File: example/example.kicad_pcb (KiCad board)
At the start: 4 copper layers, 80 x 49 mm, 124 parts, among them J1 USB_B_Micro, J2 Conn_02x10_Odd_Even, J3 Conn_02x10_Odd_Even, J4 Conn_01x02, U1 CY7C68013A-56LTX, U10 DAC081C081CIMK, U11 TPS73101DBV, U12 ADC081C021CIMM, U13 DAC081C081CIMK, U14 TPS73101DBV, U15 TPD3S014, U2 CAT24M01W, U3 CAT24C256W, U4 ICE40UP5K-SG48ITR, U5 FXMA108BQX, U6 FXMA108BQX, U7 LM3880MF-1AF, U8 MIC5355-S4YMME, U9 ADC081C021CIMM, Y1 24M

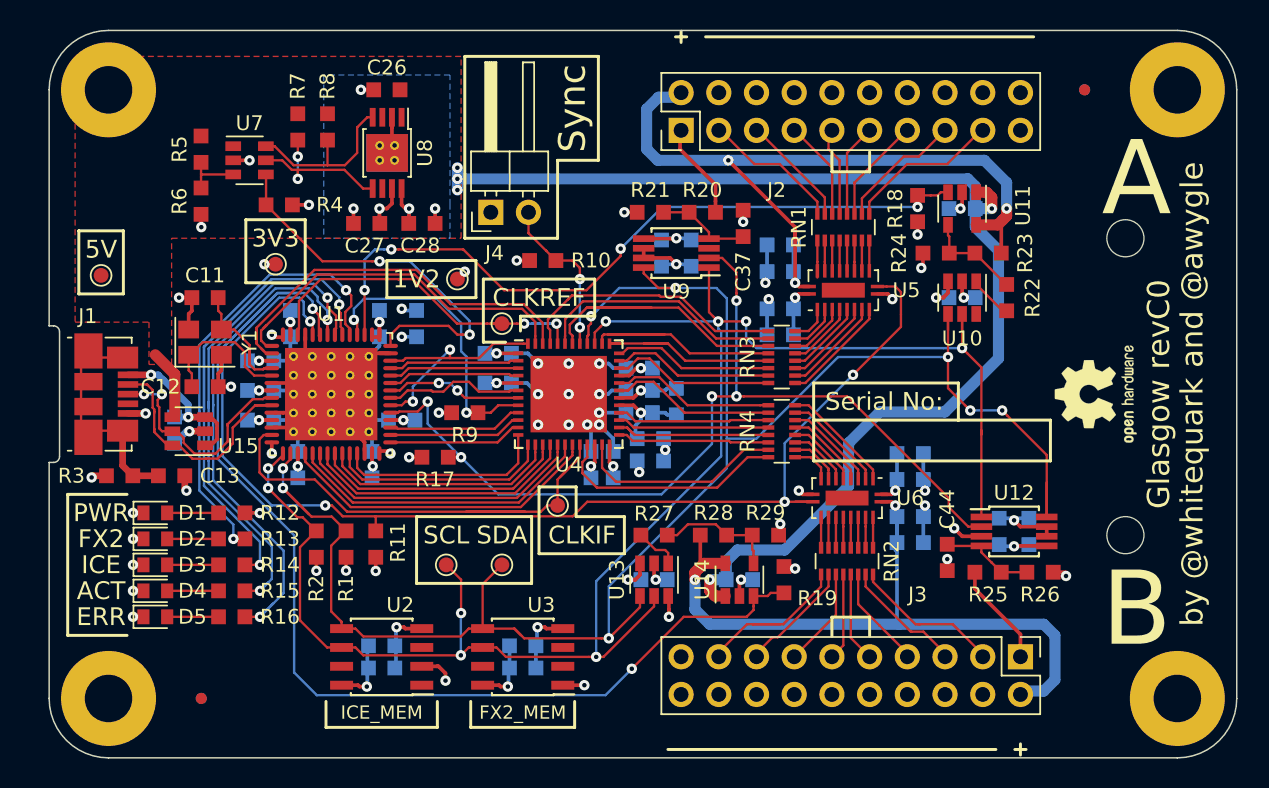
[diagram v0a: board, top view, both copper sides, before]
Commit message: Add files via upload
Updated to the current version of Glasgow.
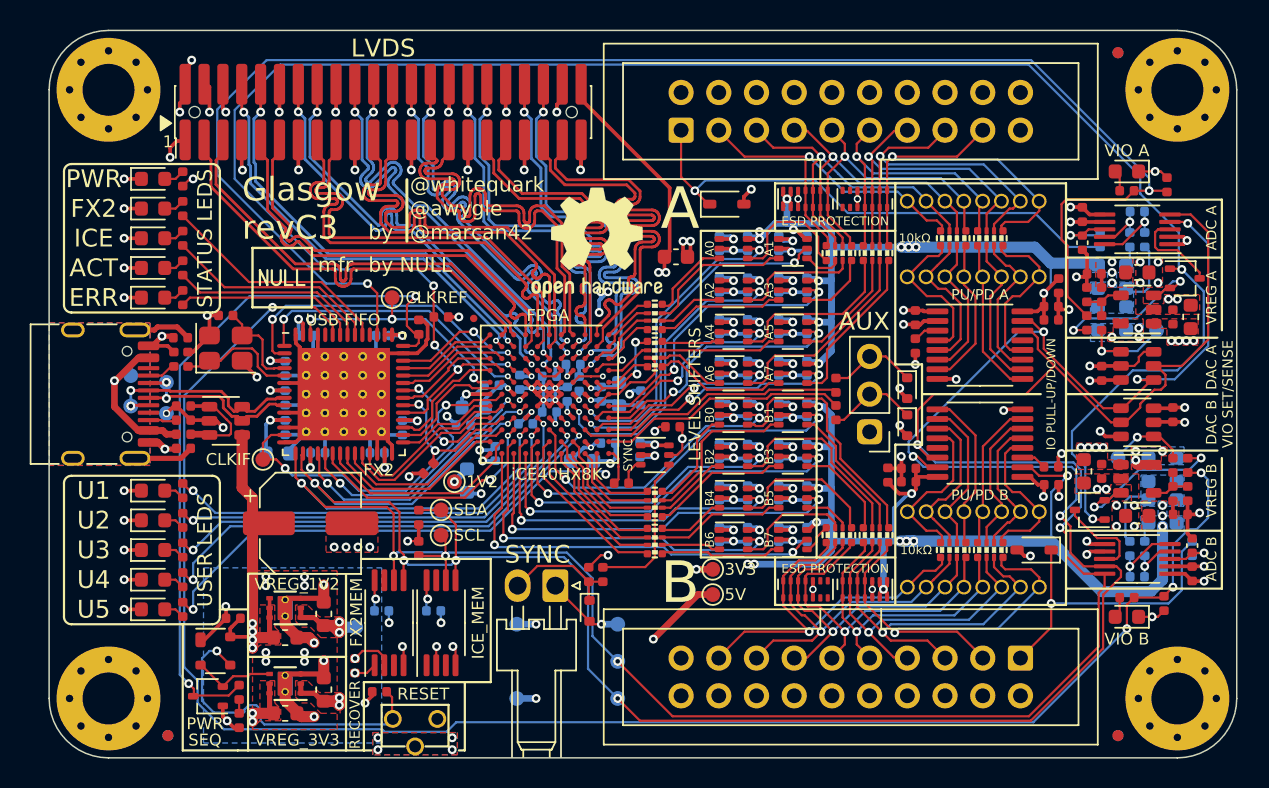
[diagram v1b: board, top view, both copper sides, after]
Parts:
- removed MK5, MK6: Mounting_Hole, MountingHole:MountingHole_2.5mm
- removed the REF** at (120.5, 95.5)
- added C48: u1, Capacitor_SMD:C_0402_1005Metric, B.Cu at (99.2, 93.8)
- added C49: u1, Capacitor_SMD:C_0402_1005Metric, B.Cu at (101.0, 85.3)
- added C50: u1, Capacitor_SMD:C_0402_1005Metric, B.Cu at (101.0, 88.2)
- added C51: u1, Capacitor_SMD:C_0402_1005Metric, B.Cu at (101.0, 91.0)
- added C52: u1, Capacitor_SMD:C_0402_1005Metric, B.Cu at (101.0, 93.8)
- added C53: 4u7, Capacitor_SMD:C_0603_1608Metric, F.Cu at (123.3, 103.7)
- added C54: u1, Capacitor_SMD:C_0402_1005Metric, F.Cu at (117.5, 89.6)
- added C55: u1, Capacitor_SMD:C_0402_1005Metric, F.Cu at (119.6, 83.4)
- added C56: u1, Capacitor_SMD:C_0402_1005Metric, F.Cu at (120.9, 94.1)
- added C57: u1, Capacitor_SMD:C_0402_1005Metric, F.Cu at (120.4, 87.4)
- added C58: u1, Capacitor_SMD:C_0402_1005Metric, B.Cu at (123.3, 83.2)
- added C59: u1, Capacitor_SMD:C_0402_1005Metric, F.Cu at (125.7, 90.3)
- added C60: u1, Capacitor_SMD:C_0402_1005Metric, B.Cu at (95.2, 96.5)
- added C61: u1, Capacitor_SMD:C_0402_1005Metric, B.Cu at (95.2, 99.3)
- added C62: u1, Capacitor_SMD:C_0402_1005Metric, B.Cu at (95.2, 102.2)
- added C63: u1, Capacitor_SMD:C_0402_1005Metric, B.Cu at (95.2, 105.0)
- added C64: u1, Capacitor_SMD:C_0402_1005Metric, B.Cu at (97.0, 96.5)
- added C65: u1, Capacitor_SMD:C_0402_1005Metric, B.Cu at (97.0, 99.3)
- added C66: u1, Capacitor_SMD:C_0402_1005Metric, B.Cu at (97.0, 102.2)
- added C67: u1, Capacitor_SMD:C_0402_1005Metric, B.Cu at (97.0, 105.0)
- added C68: u1, Capacitor_SMD:C_0402_1005Metric, B.Cu at (99.2, 96.5)
- added C69: u1, Capacitor_SMD:C_0402_1005Metric, B.Cu at (99.2, 99.3)
- added C70: u1, Capacitor_SMD:C_0402_1005Metric, B.Cu at (99.2, 102.2)
- added C71: u1, Capacitor_SMD:C_0402_1005Metric, B.Cu at (99.2, 105.0)
- added C72: u1, Capacitor_SMD:C_0402_1005Metric, B.Cu at (101.0, 96.5)
- added C73: u1, Capacitor_SMD:C_0402_1005Metric, B.Cu at (101.0, 99.3)
- added C74: u1, Capacitor_SMD:C_0402_1005Metric, B.Cu at (101.0, 102.2)
- added C75: u1, Capacitor_SMD:C_0402_1005Metric, B.Cu at (101.0, 105.0)
- added C76: 4u7, Capacitor_SMD:C_0603_1608Metric, B.Cu at (78.6, 96.4)
- added C77: u1, Capacitor_SMD:C_0402_1005Metric, B.Cu at (84.9, 95.5)
- added C78: u1, Capacitor_SMD:C_0402_1005Metric, B.Cu at (79.8, 94.9)
- added C79: u1, Capacitor_SMD:C_0402_1005Metric, B.Cu at (87.2, 95.5)
- added C80: 4u7, Capacitor_SMD:C_0603_1608Metric, B.Cu at (88.4, 95.5)
- added C81: u1, Capacitor_SMD:C_0402_1005Metric, B.Cu at (80.0, 99.5)
- added C82: 4u7, Capacitor_SMD:C_0603_1608Metric, F.Cu at (126.9, 90.3)
- added C83: 4u7, Capacitor_SMD:C_0603_1608Metric, F.Cu at (123.3, 87.3)
- added C84: u1, Capacitor_SMD:C_0402_1005Metric, F.Cu at (108.3, 90.3)
- added C85: u1, Capacitor_SMD:C_0402_1005Metric, B.Cu at (89.8, 99.2)
- added C86: 4u7, Capacitor_SMD:C_0603_1608Metric, F.Cu at (65.9, 111.9)
- added C87: 150u, Capacitor_SMD:CP_Elec_6.3x5.9, F.Cu at (67.6, 104.2)
- added C88: u1, Capacitor_SMD:C_0402_1005Metric, F.Cu at (74.9, 91.0)
- added C89: u1, Capacitor_SMD:C_0402_1005Metric, F.Cu at (72.2, 115.5)
- added C90: 1n 50V C0G, Capacitor_SMD:C_0402_1005Metric, F.Cu at (127.0, 105.7)
- added C91: 1n 50V C0G, Capacitor_SMD:C_0402_1005Metric, F.Cu at (119.6, 85.3)
- added C92: 4u7, Capacitor_SMD:C_0603_1608Metric, F.Cu at (92.2, 86.2)
- added D10: BLU, LED_SMD:LED_0603_1608Metric, F.Cu at (57.0, 110.0)
- added D11: ESD5Z5.0T1G, Glasgow:D_SOD-523, F.Cu at (86.4, 110.1)
- added D12: ESD5Z5.0T1G, Glasgow:D_SOD-523, F.Cu at (107.8, 97.6)
- added D13: ESD5Z5.0T1G, Glasgow:D_SOD-523, F.Cu at (107.8, 95.1)
- added D14: GRN, LED_SMD:LED_0603_1608Metric, F.Cu at (122.6, 110.5)
- added D15: GRN, LED_SMD:LED_0603_1608Metric, F.Cu at (122.6, 80.5)
- added D16: CDSOD323-T36S, Glasgow:D_SOD-323, F.Cu at (116.3, 106.0)
- added D17: CDSOD323-T36S, Glasgow:D_SOD-323, F.Cu at (95.7, 82.7)
- added D18: BAT54CW, Glasgow:SOT-323_SC-70, F.Cu at (120.1, 103.3)
- added D19: BAT54CW, Glasgow:SOT-323_SC-70, F.Cu at (126.5, 87.7)
- added D20: SP3012-06UTG, Glasgow:UDFN-14_3.5x1.35mm_P0.5mm, F.Cu at (105.0, 108.7)
- added D21: SP3012-06UTG, Glasgow:UDFN-14_3.5x1.35mm_P0.5mm, F.Cu at (101.0, 108.7)
- added D22: SP3012-06UTG, Glasgow:UDFN-14_3.5x1.35mm_P0.5mm, F.Cu at (101.0, 82.3)
- added D23: SP3012-06UTG, Glasgow:UDFN-14_3.5x1.35mm_P0.5mm, F.Cu at (105.0, 82.3)
- added D24: BAT54AW, Glasgow:SOT-323_SC-70, F.Cu at (60.7, 115.8)
- added D6: BLU, LED_SMD:LED_0603_1608Metric, F.Cu at (57.0, 102.0)
- added D7: PNK, LED_SMD:LED_0603_1608Metric, F.Cu at (57.0, 104.0)
- added D8: WHT, LED_SMD:LED_0603_1608Metric, F.Cu at (57.0, 106.0)
- added D9: PNK, LED_SMD:LED_0603_1608Metric, F.Cu at (57.0, 108.0)
- added FB1: 600R, 0.5A, Inductor_SMD:L_0402_1005Metric, F.Cu at (59.0, 98.2)
- added FID3: Fiducial_0.75mm_Mask1.5mm, Fiducial:Fiducial_0.75mm_Mask1.5mm, F.Cu at (122.0, 118.5)
- added FID6: Fiducial_0.75mm_Mask1.5mm, Fiducial:Fiducial_0.75mm_Mask1.5mm, B.Cu at (122.0, 118.5)
- added FID8: Fiducial_0.5mm_Dia_1mm_Outer, Fiducial:Fiducial_0.5mm_Dia_1mm_Outer, F.Cu at (78.6, 90.4)
- added J10: AUX, Connector_PinHeader_2.54mm:PinHeader_1x03_P2.54mm_Vertical, F.Cu at (105.3, 98.0)
- added J5: PinHeader_2x22_P1.27mm, Glasgow:PinHeader_2x22_P1.27mm_Vertical__SMD, F.Cu at (72.5, 76.5)
- added J6: Conn_01x08, Glasgow:PinSocket_1x08_P1.27mm_Vertical_DNP, F.Cu at (116.7, 108.5)
- added J7: Conn_01x08, Glasgow:PinSocket_1x08_P1.27mm_Vertical_DNP, F.Cu at (116.7, 103.4)
- added J8: Conn_01x08, Glasgow:PinSocket_1x08_P1.27mm_Vertical_DNP, F.Cu at (107.8, 82.5)
- added J9: Conn_01x08, Glasgow:PinSocket_1x08_P1.27mm_Vertical_DNP, F.Cu at (107.8, 87.6)
- added NONO_HANA: MECHOKKU, Glasgow:nono_hana_lines, B.Cu at (73.8, 82.5)
- added R31: 100R, Resistor_SMD:R_0402_1005Metric, B.Cu at (77.9, 97.6)
- added R32: 100R, Resistor_SMD:R_0402_1005Metric, B.Cu at (89.8, 95.8)
- added R33: 49k9, Resistor_SMD:R_0402_1005Metric, F.Cu at (120.9, 90.7)
- added R34: 59k, Resistor_SMD:R_0402_1005Metric, F.Cu at (120.9, 88.8)
- added R35: 24k3, Resistor_SMD:R_0402_1005Metric, F.Cu at (119.9, 88.8)
- added R36: 10k, Resistor_SMD:R_0402_1005Metric, F.Cu at (117.5, 100.4)
- added R37: 10k, Resistor_SMD:R_0402_1005Metric, F.Cu at (108.3, 92.2)
- added R38: 47R, Resistor_SMD:R_0402_1005Metric, F.Cu at (87.3, 107.7)
- added R39: 47R, Resistor_SMD:R_0402_1005Metric, F.Cu at (103.0, 96.8)
- added R40: DNP, Glasgow:R_0402_1005Metric_DNP, F.Cu at (70.6, 113.8)
- added R41: 2k2, Resistor_SMD:R_0402_1005Metric, F.Cu at (107.9, 100.5)
- added R42: 2k2, Resistor_SMD:R_0402_1005Metric, F.Cu at (117.5, 90.5)
- added R43: 47R, Resistor_SMD:R_0402_1005Metric, F.Cu at (103.0, 94.9)
- added R44: 10k, Resistor_SMD:R_0402_1005Metric, F.Cu at (86.3, 107.7)
- added R45: 47R, Resistor_SMD:R_0402_1005Metric, F.Cu at (88.5, 101.5)
- added R46: 20k, Resistor_SMD:R_0402_1005Metric, F.Cu at (122.6, 109.2)
- added R47: 20k, Resistor_SMD:R_0402_1005Metric, F.Cu at (122.6, 81.8)
- added R48: 0R15, Resistor_SMD:R_0603_1608Metric, B.Cu at (124.0, 103.4)
- added R49: 0R15, Resistor_SMD:R_0603_1608Metric, B.Cu at (122.5, 87.6)
- added R50: DNP, Glasgow:R_0603_1608Metric_DNP, B.Cu at (126.0, 103.4)
- added R51: DNP, Glasgow:R_0603_1608Metric_DNP, B.Cu at (120.7, 87.6)
- added R52: 5k1, Resistor_SMD:R_0402_1005Metric, F.Cu at (59.0, 97.2)
- added R53: 5k1, Resistor_SMD:R_0402_1005Metric, F.Cu at (58.4, 93.2)
- added R54: 4R7, Resistor_SMD:R_0402_1005Metric, B.Cu at (122.8, 85.1)
- added R55: 10k, Resistor_SMD:R_0402_1005Metric, F.Cu at (119.9, 90.7)
- added R56: 0R33, Resistor_SMD:R_0603_1608Metric, B.Cu at (122.5, 90.4)
- added R57: 2k2, Resistor_SMD:R_0402_1005Metric, F.Cu at (106.5, 101.0)
- added R58: 2k2, Resistor_SMD:R_0402_1005Metric, F.Cu at (118.0, 88.2)
- added R59: 470, Resistor_SMD:R_0402_1005Metric, B.Cu at (127.0, 105.9)
- added R60: 470, Resistor_SMD:R_0402_1005Metric, B.Cu at (120.8, 85.1)
- added REF**: OSHW-Logo2_9.8x8mm_SilkScreen, Symbol:OSHW-Logo2_9.8x8mm_SilkScreen, F.Cu at (86.9, 85.3)
- added REF**: null_Logo_SilkS_4mm, Glasgow:null_Logo_SilkS_4mm, F.Cu at (65.7, 87.7)
- added REF**: Tab, kikit:Tab, F.Cu at (120.0, 70.5)
- added REF**: Tab, kikit:Tab, F.Cu at (60.0, 120.5)
- added REF**: Tab, kikit:Tab, F.Cu at (60.0, 70.6)
- added REF**: Tab, kikit:Tab, F.Cu at (120.0, 120.5)
- added REF**: null_Logo_SilkS_6mm, Glasgow:null_Logo_SilkS_6mm, B.Cu at (59.5, 107.0)
- added RN10: 33R, Glasgow:R_Array_Convex_4x0402, F.Cu at (105.7, 86.0)
- added RN11: 10k, Glasgow:R_Array_Convex_4x0402, F.Cu at (110.9, 85.0)
- added RN12: 10k, Glasgow:R_Array_Convex_4x0402, F.Cu at (113.4, 85.0)
- added RN5: 10k, Glasgow:R_Array_Convex_4x0402, F.Cu at (113.4, 106.0)
- added RN6: 10k, Glasgow:R_Array_Convex_4x0402, F.Cu at (110.9, 106.0)
- added RN7: 33R, Glasgow:R_Array_Convex_4x0402, F.Cu at (90.8, 90.3)
- added RN8: 33R, Glasgow:R_Array_Convex_4x0402, F.Cu at (90.8, 92.8)
- added RN9: 33R, Glasgow:R_Array_Convex_4x0402, F.Cu at (103.2, 86.0)
- added SW1: RST, Glasgow:SW_Tactile_SPST_Angled_TC-1109DE, F.Cu at (74.7, 117.4)
- added TP10: SDA, TestPoint:TestPoint_Pad_D1.0mm, B.Cu at (88.3, 116.0)
- added TP11: SCL, TestPoint:TestPoint_Pad_D1.0mm, B.Cu at (88.3, 113.5)
- added TP12: GND, TestPoint:TestPoint_Pad_D1.0mm, B.Cu at (88.3, 111.0)
- added TP13: VBUS, TestPoint:TestPoint_Pad_D1.0mm, B.Cu at (55.5, 94.2)
- added TP14: USBGND, TestPoint:TestPoint_Pad_D1.0mm, B.Cu at (57.9, 96.8)
- added TP15: USBDP, TestPoint:TestPoint_Pad_D1.0mm, B.Cu at (55.5, 96.3)
- added TP16: USBDM, TestPoint:TestPoint_Pad_D1.0mm, B.Cu at (57.9, 94.7)
- added TP17: 1V2, TestPoint:TestPoint_Pad_D1.0mm, B.Cu at (70.7, 111.2)
- added TP18: VDAC, TestPoint:TestPoint_Pad_D1.0mm, B.Cu at (122.0, 99.8)
- added TP19: VDAC, TestPoint:TestPoint_Pad_D1.0mm, B.Cu at (124.6, 91.2)
- added TP8: 5V, TestPoint:TestPoint_Pad_D1.0mm, B.Cu at (81.5, 116.0)
- added TP9: 3V3, TestPoint:TestPoint_Pad_D1.0mm, B.Cu at (81.5, 111.0)
- added U16: SN74LVC1T45DCKR, Glasgow:SOT-363_SC-70-6, F.Cu at (100.1, 88.5)
- added U17: SN74LVC1T45DCKR, Glasgow:SOT-363_SC-70-6, F.Cu at (100.1, 91.3)
- added U18: SN74LVC1T45DCKR, Glasgow:SOT-363_SC-70-6, F.Cu at (100.1, 94.1)
- added U19: PCA6408APW, Package_SO:TSSOP-16_4.4x5mm_P0.65mm, F.Cu at (112.7, 92.2)
- added U20: DAC081C081CIMK, Glasgow:SOT-23-6, F.Cu at (123.3, 93.6)
- added U21: INA233, Glasgow:VSSOP-10_3x3mm_P0.5mm, F.Cu at (123.3, 84.4)
- added U22: SN74LVC1T45DCKR, Glasgow:SOT-363_SC-70-6, F.Cu at (96.1, 96.9)
- added U23: SN74LVC1T45DCKR, Glasgow:SOT-363_SC-70-6, F.Cu at (96.1, 99.7)
- added U24: SN74LVC1T45DCKR, Glasgow:SOT-363_SC-70-6, F.Cu at (96.1, 102.5)
- added U25: SN74LVC1T45DCKR, Glasgow:SOT-363_SC-70-6, F.Cu at (96.1, 105.3)
- added U26: SN74LVC1T45DCKR, Glasgow:SOT-363_SC-70-6, F.Cu at (100.1, 96.9)
- added U27: SN74LVC1T45DCKR, Glasgow:SOT-363_SC-70-6, F.Cu at (100.1, 99.7)
- added U28: SN74LVC1T45DCKR, Glasgow:SOT-363_SC-70-6, F.Cu at (100.1, 102.5)
- added U29: SN74LVC1T45DCKR, Glasgow:SOT-363_SC-70-6, F.Cu at (100.1, 105.3)
- added U30: ICE40HX8K-BG121, Package_BGA:BGA-121_9.0x9.0mm_Layout11x11_P0.8mm_Ball0.4mm_Pad0.35mm_NSMD, F.Cu at (83.7, 95.5)
- added U31: TPS73101DBV, Glasgow:SOT-23-5, F.Cu at (123.3, 89.8)
- added U32: SN74LVC1T45DCKR, Glasgow:SOT-363_SC-70-6, F.Cu at (90.8, 99.6)
- added U36: TLV73312PQDRVR, Glasgow:DFN-6-1EP_2x2mm_P0.65mm_EP1x1.6mm_ThermalVias, F.Cu at (65.9, 109.9)
- C1, C14, C19, C26, C27, C28: footprint Capacitor_SMD:C_0603_1608Metric_Pad0.99x1.00mm_HandSolder -> Capacitor_SMD:C_0603_1608Metric
- C10, C13, C15, C17, C2, C20, C21, C23, C24, C25, C3, C33, C35, C36, C38, C4, C40, C42, C43, C47, C5, C6, C7, C9: footprint Capacitor_SMD:C_0603_1608Metric_Pad0.99x1.00mm_HandSolder -> Capacitor_SMD:C_0402_1005Metric
- C11, C12: value 18p -> 9p; footprint Capacitor_SMD:C_0603_1608Metric_Pad0.99x1.00mm_HandSolder -> Capacitor_SMD:C_0402_1005Metric
- C16, C29, C46: value 4u7 -> u1; footprint Capacitor_SMD:C_0603_1608Metric_Pad0.99x1.00mm_HandSolder -> Capacitor_SMD:C_0402_1005Metric; moved to F.Cu
- C18, C34, C39, C41: value 4u7 -> u1; footprint Capacitor_SMD:C_0603_1608Metric_Pad0.99x1.00mm_HandSolder -> Capacitor_SMD:C_0402_1005Metric
- C22, C30, C32, C45, C8: footprint Capacitor_SMD:C_0603_1608Metric_Pad0.99x1.00mm_HandSolder -> Capacitor_SMD:C_0402_1005Metric; moved to F.Cu
- C31: footprint Capacitor_SMD:C_0603_1608Metric_Pad0.99x1.00mm_HandSolder -> Capacitor_SMD:C_0603_1608Metric; moved to F.Cu
- C37, C44: value 12n -> u1; footprint Capacitor_SMD:C_0603_1608Metric_Pad0.99x1.00mm_HandSolder -> Capacitor_SMD:C_0402_1005Metric; moved to B.Cu
- D1, D5: footprint LED_SMD:LED_0603_1608Metric_Pad0.82x1.00mm_HandSolder -> LED_SMD:LED_0603_1608Metric
- D2: value GRN -> WHT; footprint LED_SMD:LED_0603_1608Metric_Pad0.82x1.00mm_HandSolder -> LED_SMD:LED_0603_1608Metric
- D3: value GRN -> BLU; footprint LED_SMD:LED_0603_1608Metric_Pad0.82x1.00mm_HandSolder -> LED_SMD:LED_0603_1608Metric
- D4: value YEL -> ORA; footprint LED_SMD:LED_0603_1608Metric_Pad0.82x1.00mm_HandSolder -> LED_SMD:LED_0603_1608Metric
- FID1, FID2: value Fiducial_0.75mm_Dia_1.5mm_Outer -> Fiducial_0.75mm_Mask1.5mm; footprint Fiducial:Fiducial_0.75mm_Dia_1.5mm_Outer -> Fiducial:Fiducial_0.75mm_Mask1.5mm
- FID4: renamed from FID1; value Fiducial_0.75mm_Dia_1.5mm_Outer -> Fiducial_0.75mm_Mask1.5mm; footprint Fiducial:Fiducial_0.75mm_Dia_1.5mm_Outer -> Fiducial:Fiducial_0.75mm_Mask1.5mm
- FID5: renamed from FID4; value Fiducial_0.75mm_Dia_1.5mm_Outer -> Fiducial_0.75mm_Mask1.5mm; footprint Fiducial:Fiducial_0.75mm_Dia_1.5mm_Outer -> Fiducial:Fiducial_0.75mm_Mask1.5mm
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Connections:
- net /IOBufferB/VFB renamed /IO_Banks/IO_Buffer_B/VFB
- net Net-(R27-Pad1) renamed /IO_Banks/IO_Buffer_B/VDAC
- C14 pad 1: +3V3 -> +1V2
- C16 pad 1: +3V3 -> +5V
- C18 pad 1: /VCCPLL -> +1V2
- C26 pad 1: +5V -> GND
- C26 pad 2: GND -> +5V
- C29 pad 1: +3V3 -> /IO_Banks/VIOB
- C31 pad 1: +3V3 -> +5V
- C33 pad 1: /VCCPLL -> /IO_Banks/VIO_AUX
- C37 pad 1: /IOBufferA/VSAMP -> +3V3
- C38 pad 1: +5V -> /IO_Banks/VIOA
- C39 pad 1: /IOBufferA/VIO -> /IO_Banks/VIOA
- C40 pad 1: /IOBufferA/VIO -> /IO_Banks/VIOA
- C41 pad 1: +3V3 -> /IO_Banks/VIOA
- C44 pad 1: /IOBufferB/VSAMP -> Net-(U12-Vin-)
- C44 pad 2: GND -> Net-(U12-Vin+)
- C46 pad 1: /IOBufferB/VIO -> /IO_Banks/VIOB
- C47 pad 1: /IOBufferB/VIO -> +3V3
- J2 pad 1: /IOBufferA/VSENSE -> /IO_Banks/IO_Buffer_A/VSENSE
- J2 pad 11: /IOBufferA/Z4 -> /IO_Banks/IO_Buffer_A/Z4
- J2 pad 13: /IOBufferA/Z5 -> /IO_Banks/IO_Buffer_A/Z5
- J2 pad 15: /IOBufferA/Z6 -> /IO_Banks/IO_Buffer_A/Z6
- J2 pad 17: /IOBufferA/Z7 -> /IO_Banks/IO_Buffer_A/Z7
- J2 pad 19: Net-(J2-Pad19) -> unconnected-(J2-Pin_19-Pad19)
- J2 pad 2: /IOBufferA/VIO -> /IO_Banks/VIOA
- J2 pad 20: GND -> unconnected-(J2-Pin_20-Pad20)
- J2 pad 3: /IOBufferA/Z0 -> /IO_Banks/IO_Buffer_A/Z0
- J2 pad 5: /IOBufferA/Z1 -> /IO_Banks/IO_Buffer_A/Z1
- J2 pad 7: /IOBufferA/Z2 -> /IO_Banks/IO_Buffer_A/Z2
- J2 pad 9: /IOBufferA/Z3 -> /IO_Banks/IO_Buffer_A/Z3
- J3 pad 1: /IOBufferB/VSENSE -> /IO_Banks/IO_Buffer_B/VSENSE
- J3 pad 11: /IOBufferB/Z4 -> /IO_Banks/IO_Buffer_B/Z4
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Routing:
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- added copper zone on F.Cu, net +1V2
- added copper zone on In2.Cu, net +1V2
- added copper zone on F.Cu, net +3V3
- added copper zone on B.Cu, net /IO_Banks/IO_Buffer_A/ISNS_H
- added copper zone on B.Cu, net /IO_Banks/IO_Buffer_B/ISNS_H
- added copper zone on B.Cu, net /IO_Banks/VIOA
- added copper zone on F.Cu, net /IO_Banks/VIOA
- added copper zone on B.Cu, net /IO_Banks/VIOB
- added copper zone on F.Cu, net /IO_Banks/VIOB
- added copper zone on B.Cu, net /SHLD
- added copper zone on F.Cu, net /SHLD
- added copper zone on In1.Cu, net /SHLD
- added copper zone on In2.Cu, net /SHLD
- added copper zone on B.Cu, net /SWSH
- added copper zone on F.Cu, net /SWSH
- added copper zone on In1.Cu, net /SWSH
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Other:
- outline, holes or cut-outs redrawn
- net class Default removed
- net class Power removed
- board text added: "0"
- board text added: "1"
- board text added: "10kΩ"
- board text added: "2"
- board text added: "3"
- board text added: "4"
- board text added: "5"
- board text added: "6"
- board text added: "7"
- board text added: "@whitequark @awygle @marcan42"
- board text added: "A 0"
- board text added: "A 1"
- board text added: "A 2"
- board text added: "A 3"
- board text added: "A 4"
- board text added: "A 5"
- board text added: "A 6"
- board text added: "A 7"
- board text added: "A0"
- board text added: "A1"
- board text added: "A2"
- board text added: "A3"
- board text added: "A4"
- board text added: "A5"
- board text added: "A6"
- board text added: "A7"
- board text added: "ADC A"
- board text added: "ADC B"
- board text added: "AUX"
- board text added: "B 0"
- board text added: "B 1"
- board text added: "B 2"
- board text added: "B 3"
- board text added: "B 4"
- board text added: "B 5"
- board text added: "B 6"
- board text added: "B 7"
- board text added: "B0"
- board text added: "B1"
- board text added: "B2"
- board text added: "B3"
- board text added: "B4"
- board text added: "B5"
- board text added: "B6"
- board text added: "B7"
- board text added: "Caution: Check washer & screw size for conflicts with LVDS connector"
- board text added: "D+"
- board text added: "D-"
- board text added: "DAC A"
- board text added: "DAC B"
- board text added: "ESD PROTECTION"
- board text added: "FPGA"
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
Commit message: Revert "Add files via upload"
This reverts commit 0c712be9a306c6d0f1b8a2063bd4b359c656085a.
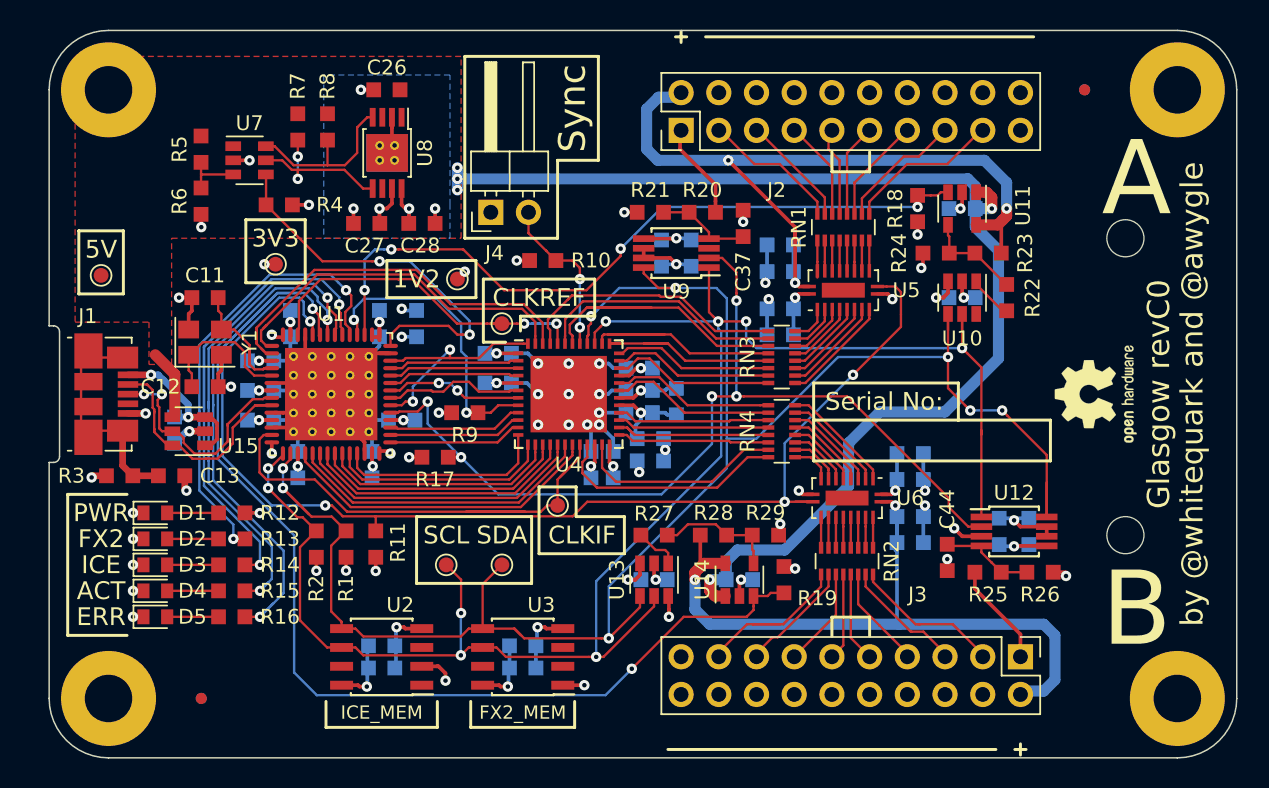
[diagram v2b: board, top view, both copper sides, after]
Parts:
- removed C48, C49, C50, C51, C52, C54, C55, C56, C57, C58, C59, C60, C61, C62, C63, C64, C65, C66, C67, C68, C69, C70, C71, C72, C73, C74, C75, C77, C78, C79, C81, C84, C85, C88, C89: u1, Capacitor_SMD:C_0402_1005Metric
- removed C53, C76, C80, C82, C83, C86, C92: 4u7, Capacitor_SMD:C_0603_1608Metric
- removed C87: 150u, Capacitor_SMD:CP_Elec_6.3x5.9
- removed C90, C91: 1n 50V C0G, Capacitor_SMD:C_0402_1005Metric
- removed D10, D6: BLU, LED_SMD:LED_0603_1608Metric
- removed D11, D12, D13: ESD5Z5.0T1G, Glasgow:D_SOD-523
- removed D14, D15: GRN, LED_SMD:LED_0603_1608Metric
- removed D16, D17: CDSOD323-T36S, Glasgow:D_SOD-323
- removed D18, D19: BAT54CW, Glasgow:SOT-323_SC-70
- removed D20, D21, D22, D23: SP3012-06UTG, Glasgow:UDFN-14_3.5x1.35mm_P0.5mm
- removed D24: BAT54AW, Glasgow:SOT-323_SC-70
- removed D7, D9: PNK, LED_SMD:LED_0603_1608Metric
- removed D8: WHT, LED_SMD:LED_0603_1608Metric
- removed FB1: 600R, 0.5A, Inductor_SMD:L_0402_1005Metric
- removed FID3, FID6: Fiducial_0.75mm_Mask1.5mm, Fiducial:Fiducial_0.75mm_Mask1.5mm
- removed FID8: Fiducial_0.5mm_Dia_1mm_Outer, Fiducial:Fiducial_0.5mm_Dia_1mm_Outer
- removed J10: AUX, Connector_PinHeader_2.54mm:PinHeader_1x03_P2.54mm_Vertical
- removed J5: PinHeader_2x22_P1.27mm, Glasgow:PinHeader_2x22_P1.27mm_Vertical__SMD
- removed J6, J7, J8, J9: Conn_01x08, Glasgow:PinSocket_1x08_P1.27mm_Vertical_DNP
- removed NONO_HANA: MECHOKKU, Glasgow:nono_hana_lines
- removed R31, R32: 100R, Resistor_SMD:R_0402_1005Metric
- removed R33: 49k9, Resistor_SMD:R_0402_1005Metric
- removed R34: 59k, Resistor_SMD:R_0402_1005Metric
- removed R35: 24k3, Resistor_SMD:R_0402_1005Metric
- removed R36, R37, R44, R55: 10k, Resistor_SMD:R_0402_1005Metric
- removed R38, R39, R43, R45: 47R, Resistor_SMD:R_0402_1005Metric
- removed R40: DNP, Glasgow:R_0402_1005Metric_DNP
- removed R41, R42, R57, R58: 2k2, Resistor_SMD:R_0402_1005Metric
- removed R46, R47: 20k, Resistor_SMD:R_0402_1005Metric
- removed R48, R49: 0R15, Resistor_SMD:R_0603_1608Metric
- removed R50, R51: DNP, Glasgow:R_0603_1608Metric_DNP
- removed R52, R53: 5k1, Resistor_SMD:R_0402_1005Metric
- removed R54: 4R7, Resistor_SMD:R_0402_1005Metric
- removed R56: 0R33, Resistor_SMD:R_0603_1608Metric
- removed R59, R60: 470, Resistor_SMD:R_0402_1005Metric
- removed the REF** at (86.9, 85.3)
- removed the REF** at (65.7, 87.7)
- removed the REF** at (120.0, 70.5)
- removed the REF** at (60.0, 120.5)
- removed the REF** at (60.0, 70.6)
- removed the REF** at (120.0, 120.5)
- removed the REF** at (59.5, 107.0)
- removed RN10, RN7, RN8, RN9: 33R, Glasgow:R_Array_Convex_4x0402
- removed RN11, RN12, RN5, RN6: 10k, Glasgow:R_Array_Convex_4x0402
- removed SW1: RST, Glasgow:SW_Tactile_SPST_Angled_TC-1109DE
- removed TP10: SDA, TestPoint:TestPoint_Pad_D1.0mm
- removed TP11: SCL, TestPoint:TestPoint_Pad_D1.0mm
- removed TP12: GND, TestPoint:TestPoint_Pad_D1.0mm
- removed TP13: VBUS, TestPoint:TestPoint_Pad_D1.0mm
- removed TP14: USBGND, TestPoint:TestPoint_Pad_D1.0mm
- removed TP15: USBDP, TestPoint:TestPoint_Pad_D1.0mm
- removed TP16: USBDM, TestPoint:TestPoint_Pad_D1.0mm
- removed TP17: 1V2, TestPoint:TestPoint_Pad_D1.0mm
- removed TP18, TP19: VDAC, TestPoint:TestPoint_Pad_D1.0mm
- removed TP8: 5V, TestPoint:TestPoint_Pad_D1.0mm
- removed TP9: 3V3, TestPoint:TestPoint_Pad_D1.0mm
- removed U16, U17, U18, U22, U23, U24, U25, U26, U27, U28, U29, U32: SN74LVC1T45DCKR, Glasgow:SOT-363_SC-70-6
- removed U19: PCA6408APW, Package_SO:TSSOP-16_4.4x5mm_P0.65mm
- removed U20: DAC081C081CIMK, Glasgow:SOT-23-6
- removed U21: INA233, Glasgow:VSSOP-10_3x3mm_P0.5mm
- removed U30: ICE40HX8K-BG121, Package_BGA:BGA-121_9.0x9.0mm_Layout11x11_P0.8mm_Ball0.4mm_Pad0.35mm_NSMD
- removed U31: TPS73101DBV, Glasgow:SOT-23-5
- removed U36: TLV73312PQDRVR, Glasgow:DFN-6-1EP_2x2mm_P0.65mm_EP1x1.6mm_ThermalVias
- added MK5: Mounting_Hole, MountingHole:MountingHole_2.5mm, F.Cu at (122.5, 105.0)
- added MK6: Mounting_Hole, MountingHole:MountingHole_2.5mm, F.Cu at (122.5, 85.0)
- added REF**: OSHW-Logo2_7.3x6mm_SilkScreen, Symbol:OSHW-Logo2_7.3x6mm_SilkScreen, F.Cu at (120.5, 95.5)
- C1, C14, C19, C26, C27, C28: footprint Capacitor_SMD:C_0603_1608Metric -> Capacitor_SMD:C_0603_1608Metric_Pad0.99x1.00mm_HandSolder
- C10, C13, C15, C17, C2, C20, C21, C23, C24, C25, C3, C33, C35, C36, C38, C4, C40, C42, C43, C47, C5, C6, C7, C9: footprint Capacitor_SMD:C_0402_1005Metric -> Capacitor_SMD:C_0603_1608Metric_Pad0.99x1.00mm_HandSolder
- C11, C12: value 9p -> 18p; footprint Capacitor_SMD:C_0402_1005Metric -> Capacitor_SMD:C_0603_1608Metric_Pad0.99x1.00mm_HandSolder
- C16, C29, C46: value u1 -> 4u7; footprint Capacitor_SMD:C_0402_1005Metric -> Capacitor_SMD:C_0603_1608Metric_Pad0.99x1.00mm_HandSolder; moved to B.Cu
- C18, C34, C39, C41: value u1 -> 4u7; footprint Capacitor_SMD:C_0402_1005Metric -> Capacitor_SMD:C_0603_1608Metric_Pad0.99x1.00mm_HandSolder
- C22, C30, C32, C45, C8: footprint Capacitor_SMD:C_0402_1005Metric -> Capacitor_SMD:C_0603_1608Metric_Pad0.99x1.00mm_HandSolder; moved to B.Cu
- C31: footprint Capacitor_SMD:C_0603_1608Metric -> Capacitor_SMD:C_0603_1608Metric_Pad0.99x1.00mm_HandSolder; moved to B.Cu
- C37, C44: value u1 -> 12n; footprint Capacitor_SMD:C_0402_1005Metric -> Capacitor_SMD:C_0603_1608Metric_Pad0.99x1.00mm_HandSolder; moved to F.Cu
- D1, D5: footprint LED_SMD:LED_0603_1608Metric -> LED_SMD:LED_0603_1608Metric_Pad0.82x1.00mm_HandSolder
- D2: value WHT -> GRN; footprint LED_SMD:LED_0603_1608Metric -> LED_SMD:LED_0603_1608Metric_Pad0.82x1.00mm_HandSolder
- D3: value BLU -> GRN; footprint LED_SMD:LED_0603_1608Metric -> LED_SMD:LED_0603_1608Metric_Pad0.82x1.00mm_HandSolder
- D4: value ORA -> YEL; footprint LED_SMD:LED_0603_1608Metric -> LED_SMD:LED_0603_1608Metric_Pad0.82x1.00mm_HandSolder
- FID1: renamed from FID4; value Fiducial_0.75mm_Mask1.5mm -> Fiducial_0.75mm_Dia_1.5mm_Outer; footprint Fiducial:Fiducial_0.75mm_Mask1.5mm -> Fiducial:Fiducial_0.75mm_Dia_1.5mm_Outer
- FID1, FID2: value Fiducial_0.75mm_Mask1.5mm -> Fiducial_0.75mm_Dia_1.5mm_Outer; footprint Fiducial:Fiducial_0.75mm_Mask1.5mm -> Fiducial:Fiducial_0.75mm_Dia_1.5mm_Outer
- FID4: renamed from FID5; value Fiducial_0.75mm_Mask1.5mm -> Fiducial_0.75mm_Dia_1.5mm_Outer; footprint Fiducial:Fiducial_0.75mm_Mask1.5mm -> Fiducial:Fiducial_0.75mm_Dia_1.5mm_Outer
- J1: value USB_C_USB2.0 -> USB_B_Micro; footprint Glasgow:USB_C_Receptacle_HRO_TYPE-C-31-M-12 -> Connector_USB:USB_Micro-B_Molex_47346-0001
- J2, J3: value IDC-Header_2x10_P2.54mm -> Conn_02x10_Odd_Even; footprint Connector_IDC:IDC-Header_2x10_P2.54mm_Vertical -> Connector_PinHeader_2.54mm:PinHeader_2x10_P2.54mm_Vertical
- J4: footprint Glasgow:Molex_KK-254_1x02_P2.54mm_Horizontal -> Connector_PinHeader_2.54mm:PinHeader_1x02_P2.54mm_Horizontal
- MK1, MK2, MK3, MK4: footprint Glasgow:MountingHole_3.5mm_Pad_Via_CrtYd -> MountingHole:MountingHole_3.2mm_M3_Pad
- R1, R13, R14, R17, R2, R26, R27, R28, R29, R4, R9: footprint Resistor_SMD:R_0402_1005Metric -> Resistor_SMD:R_0603_1608Metric_Pad0.99x1.00mm_HandSolder
- R10: value 2k2 -> 390; footprint Resistor_SMD:R_0402_1005Metric -> Resistor_SMD:R_0603_1608Metric_Pad0.99x1.00mm_HandSolder
- R11: value 2k2 -> 100k; footprint Resistor_SMD:R_0402_1005Metric -> Resistor_SMD:R_0603_1608Metric_Pad0.99x1.00mm_HandSolder
- R12: value 10k -> 2k2; footprint Resistor_SMD:R_0402_1005Metric -> Resistor_SMD:R_0603_1608Metric_Pad0.99x1.00mm_HandSolder
- R15: value 1k -> 390; footprint Resistor_SMD:R_0402_1005Metric -> Resistor_SMD:R_0603_1608Metric_Pad0.99x1.00mm_HandSolder
- R16: value 1k -> 604; footprint Resistor_SMD:R_0402_1005Metric -> Resistor_SMD:R_0603_1608Metric_Pad0.99x1.00mm_HandSolder
- R18, R19: value 10k -> 100k; footprint Resistor_SMD:R_0402_1005Metric -> Resistor_SMD:R_0603_1608Metric_Pad0.99x1.00mm_HandSolder
- R20, R21: value 2k2 -> 10k; footprint Resistor_SMD:R_0402_1005Metric -> Resistor_SMD:R_0603_1608Metric_Pad0.99x1.00mm_HandSolder
- R22: value 2k2 -> 49k9; footprint Resistor_SMD:R_0402_1005Metric -> Resistor_SMD:R_0603_1608Metric_Pad0.99x1.00mm_HandSolder
- R23: value 2k2 -> 59k; footprint Resistor_SMD:R_0402_1005Metric -> Resistor_SMD:R_0603_1608Metric_Pad0.99x1.00mm_HandSolder
- R24: value 4R7 -> 24k3; footprint Resistor_SMD:R_0402_1005Metric -> Resistor_SMD:R_0603_1608Metric_Pad0.99x1.00mm_HandSolder; moved to F.Cu
- R25: value 4R7 -> 10k; footprint Resistor_SMD:R_0402_1005Metric -> Resistor_SMD:R_0603_1608Metric_Pad0.99x1.00mm_HandSolder; moved to F.Cu
- R3: value 100k -> 1M; footprint Resistor_SMD:R_0402_1005Metric -> Resistor_SMD:R_0603_1608Metric_Pad0.99x1.00mm_HandSolder
- R30: value 4R7 -> 100; footprint Resistor_SMD:R_0402_1005Metric -> Resistor_SMD:R_0603_1608Metric_Pad0.99x1.00mm_HandSolder
- R5: value 100k -> 220k; footprint Resistor_SMD:R_0402_1005Metric -> Resistor_SMD:R_0603_1608Metric_Pad0.99x1.00mm_HandSolder
- R6, R8: value DNP -> 100k; footprint Glasgow:R_0603_1608Metric_DNP -> Resistor_SMD:R_0603_1608Metric_Pad0.99x1.00mm_HandSolder; moved to F.Cu
- R7: value 0R33 -> 100k; footprint Resistor_SMD:R_0603_1608Metric -> Resistor_SMD:R_0603_1608Metric_Pad0.99x1.00mm_HandSolder; moved to F.Cu
- RN1, RN2, RN3, RN4: value 33R -> R_Pack08; footprint Glasgow:R_Array_Convex_4x0402 -> Resistor_SMD:R_Array_Convex_8x0602
- U10: value SN74LVC1T45DCKR -> DAC081C081CIMK; footprint Glasgow:SOT-363_SC-70-6 -> Package_TO_SOT_SMD:SOT-23-6
- U11: value SN74LVC1T45DCKR -> TPS73101DBV; footprint Glasgow:SOT-363_SC-70-6 -> Package_TO_SOT_SMD:SOT-23-5
- U12: value INA233 -> ADC081C021CIMM; footprint Glasgow:VSSOP-10_3x3mm_P0.5mm -> Package_SO:MSOP-8_3x3mm_P0.65mm
- U13, U15: footprint Glasgow:SOT-23-6 -> Package_TO_SOT_SMD:SOT-23-6
- U14: footprint Glasgow:SOT-23-5 -> Package_TO_SOT_SMD:SOT-23-5
- U2: value CAT24M01X -> CAT24M01W; footprint Package_SO:TSSOP-8_4.4x3mm_P0.65mm -> Package_SO:SOIC-8_3.9x4.9mm_P1.27mm
- U3: value BL24C256A-SFRC -> CAT24C256W; footprint Package_SO:TSSOP-8_4.4x3mm_P0.65mm -> Package_SO:SOIC-8_3.9x4.9mm_P1.27mm
- U4: value SN74LVC1T45DCKR -> ICE40UP5K-SG48ITR; footprint Glasgow:SOT-363_SC-70-6 -> Package_DFN_QFN:QFN-48-1EP_7x7mm_P0.5mm_EP5.15x5.15mm
- U5: value PCA6408APW -> FXMA108BQX; footprint Package_SO:TSSOP-16_4.4x5mm_P0.65mm -> Package_DFN_QFN:WQFN-20-1EP_2.5x4.5mm_P0.5mm_EP1x2.9mm
- U6: value SN74LVC1T45DCKR -> FXMA108BQX; footprint Glasgow:SOT-363_SC-70-6 -> Package_DFN_QFN:WQFN-20-1EP_2.5x4.5mm_P0.5mm_EP1x2.9mm
- U7: value APX811-40UG-7 -> LM3880MF-1AF; footprint Glasgow:SOT-143 -> Package_TO_SOT_SMD:SOT-23-6
- U8: value TLV75533PDRVR -> MIC5355-S4YMME; footprint Glasgow:DFN-6-1EP_2x2mm_P0.65mm_EP1x1.6mm_ThermalVias -> Package_SO:MSOP-8-1EP_3x3mm_P0.65mm_EP2.54x2.8mm_ThermalVias
- U9: value SN74LVC1T45DCKR -> ADC081C021CIMM; footprint Glasgow:SOT-363_SC-70-6 -> Package_SO:MSOP-8_3x3mm_P0.65mm
- Y1: footprint Glasgow:Crystal_SMD_3225-4Pin_3.2x2.5mm -> Crystals:Crystal_SMD_3225-4pin_3.2x2.5mm
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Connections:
- net /IO_Banks/IO_Buffer_B/VDAC renamed Net-(R27-Pad1)
- net /IO_Banks/IO_Buffer_B/VFB renamed /IOBufferB/VFB
- C14 pad 1: +1V2 -> +3V3
- C16 pad 1: +5V -> +3V3
- C18 pad 1: +1V2 -> /VCCPLL
- C26 pad 1: GND -> +5V
- C26 pad 2: +5V -> GND
- C29 pad 1: /IO_Banks/VIOB -> +3V3
- C31 pad 1: +5V -> +3V3
- C33 pad 1: /IO_Banks/VIO_AUX -> /VCCPLL
- C37 pad 1: +3V3 -> /IOBufferA/VSAMP
- C38 pad 1: /IO_Banks/VIOA -> +5V
- C39 pad 1: /IO_Banks/VIOA -> /IOBufferA/VIO
- C40 pad 1: /IO_Banks/VIOA -> /IOBufferA/VIO
- C41 pad 1: /IO_Banks/VIOA -> +3V3
- C44 pad 1: Net-(U12-Vin-) -> /IOBufferB/VSAMP
- C44 pad 2: Net-(U12-Vin+) -> GND
- C46 pad 1: /IO_Banks/VIOB -> /IOBufferB/VIO
- C47 pad 1: +3V3 -> /IOBufferB/VIO
- J2 pad 1: /IO_Banks/IO_Buffer_A/VSENSE -> /IOBufferA/VSENSE
- J2 pad 11: /IO_Banks/IO_Buffer_A/Z4 -> /IOBufferA/Z4
- J2 pad 13: /IO_Banks/IO_Buffer_A/Z5 -> /IOBufferA/Z5
- J2 pad 15: /IO_Banks/IO_Buffer_A/Z6 -> /IOBufferA/Z6
- J2 pad 17: /IO_Banks/IO_Buffer_A/Z7 -> /IOBufferA/Z7
- J2 pad 19: unconnected-(J2-Pin_19-Pad19) -> Net-(J2-Pad19)
- J2 pad 2: /IO_Banks/VIOA -> /IOBufferA/VIO
- J2 pad 20: unconnected-(J2-Pin_20-Pad20) -> GND
- J2 pad 3: /IO_Banks/IO_Buffer_A/Z0 -> /IOBufferA/Z0
- J2 pad 5: /IO_Banks/IO_Buffer_A/Z1 -> /IOBufferA/Z1
- J2 pad 7: /IO_Banks/IO_Buffer_A/Z2 -> /IOBufferA/Z2
- J2 pad 9: /IO_Banks/IO_Buffer_A/Z3 -> /IOBufferA/Z3
- J3 pad 1: /IO_Banks/IO_Buffer_B/VSENSE -> /IOBufferB/VSENSE
- J3 pad 11: /IO_Banks/IO_Buffer_B/Z4 -> /IOBufferB/Z4
- J3 pad 13: /IO_Banks/IO_Buffer_B/Z5 -> /IOBufferB/Z5
- J3 pad 15: /IO_Banks/IO_Buffer_B/Z6 -> /IOBufferB/Z6
- J3 pad 17: /IO_Banks/IO_Buffer_B/Z7 -> /IOBufferB/Z7
- J3 pad 19: unconnected-(J3-Pin_19-Pad19) -> Net-(J3-Pad19)
- J3 pad 2: /IO_Banks/VIOB -> /IOBufferB/VIO
- J3 pad 20: unconnected-(J3-Pin_20-Pad20) -> GND
- J3 pad 3: /IO_Banks/IO_Buffer_B/Z0 -> /IOBufferB/Z0
- J3 pad 5: /IO_Banks/IO_Buffer_B/Z1 -> /IOBufferB/Z1
- J3 pad 7: /IO_Banks/IO_Buffer_B/Z2 -> /IOBufferB/Z2
- J3 pad 9: /IO_Banks/IO_Buffer_B/Z3 -> /IOBufferB/Z3
- J4 pad 2: /IO_Banks/~{SYNC} -> /~SYNC
- R10 pad 1: Net-(U30A-IOT_219) -> /~SYNC
- R10 pad 2: GND -> +3V3
- R11 pad 1: /IO_Banks/U1 -> /~OEQ
- R11 pad 2: Net-(D6-A) -> +3V3
- R17 pad 1: /~{ALERT} -> /~ALERT
- R20 pad 1: /IO_Banks/U2 -> /IOBufferA/VSAMP
- R20 pad 2: Net-(D7-A) -> /IOBufferA/VSENSE
- R21 pad 1: /IO_Banks/U3 -> GND
- R21 pad 2: Net-(D8-A) -> /IOBufferA/VSAMP
- R22 pad 1: /IO_Banks/U4 -> Net-(R22-Pad1)
- R22 pad 2: Net-(D9-A) -> /IOBufferA/VFB
- R23 pad 1: /IO_Banks/U5 -> /IOBufferA/VFB
- R23 pad 2: Net-(D10-A) -> /IOBufferA/VIO
- R24 pad 1: /IO_Banks/IO_Buffer_B/ISNS_H -> GND
- R24 pad 2: Net-(U12-Vin+) -> /IOBufferA/VFB
- R25 pad 1: /IO_Banks/VIOB -> /IOBufferB/VSAMP
- R25 pad 2: Net-(U12-Vin-) -> /IOBufferB/VSENSE
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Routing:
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- removed copper zone on F.Cu, net +1V2
- removed copper zone on In2.Cu, net +1V2
- removed copper zone on F.Cu, net +3V3
- removed copper zone on B.Cu, net /IO_Banks/IO_Buffer_A/ISNS_H
- removed copper zone on B.Cu, net /IO_Banks/IO_Buffer_B/ISNS_H
- removed copper zone on B.Cu, net /IO_Banks/VIOA
- removed copper zone on F.Cu, net /IO_Banks/VIOA
- removed copper zone on B.Cu, net /IO_Banks/VIOB
- removed copper zone on F.Cu, net /IO_Banks/VIOB
- removed copper zone on B.Cu, net /SHLD
- removed copper zone on F.Cu, net /SHLD
- removed copper zone on In1.Cu, net /SHLD
- removed copper zone on In2.Cu, net /SHLD
- removed copper zone on B.Cu, net /SWSH
- removed copper zone on F.Cu, net /SWSH
- removed copper zone on In1.Cu, net /SWSH
- removed copper zone on F.Cu, net GND
- removed copper zone on B.Cu, net Net-(U14-OUT)
- removed copper zone on F.Cu, net Net-(U14-OUT)
- removed copper zone on B.Cu, net Net-(U31-OUT)
- removed copper zone on F.Cu, net Net-(U31-OUT)
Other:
- outline, holes or cut-outs redrawn
- net class Default added: clearance 0.15, trace_width 0.16, via_dia 0.7, via_drill 0.3
- net class Power added: clearance 0.15, trace_width 0.25, via_dia 0.7, via_drill 0.3
- board text added: "FX2_MEM"
- board text added: "Glasgow revC0"
- board text added: "Sync"
- board text added: "by @whitequark and @awygle"
- board text removed: "0"
- board text removed: "1"
- board text removed: "10kΩ"
- board text removed: "2"
- board text removed: "3"
- board text removed: "4"
- board text removed: "5"
- board text removed: "6"
- board text removed: "7"
- board text removed: "@whitequark @awygle @marcan42"
- board text removed: "A 0"
- board text removed: "A 1"
- board text removed: "A 2"
- board text removed: "A 3"
- board text removed: "A 4"
- board text removed: "A 5"
- board text removed: "A 6"
- board text removed: "A 7"
- board text removed: "A0"
- board text removed: "A1"
- board text removed: "A2"
- board text removed: "A3"
- board text removed: "A4"
- board text removed: "A5"
- board text removed: "A6"
- board text removed: "A7"
- board text removed: "ADC A"
- board text removed: "ADC B"
- board text removed: "AUX"
- board text removed: "B 0"
- board text removed: "B 1"
- board text removed: "B 2"
- board text removed: "B 3"
- board text removed: "B 4"
- board text removed: "B 5"
- board text removed: "B 6"
- board text removed: "B 7"
- board text removed: "B0"
- board text removed: "B1"
- board text removed: "B2"
- board text removed: "B3"
- board text removed: "B4"
- board text removed: "B5"
- board text removed: "B6"
- board text removed: "B7"
- board text removed: "Caution: Check washer & screw size for conflicts with LVDS connector"
- board text removed: "D+"
- board text removed: "D-"
- board text removed: "DAC A"
- board text removed: "DAC B"
- board text removed: "ESD PROTECTION"
- board text removed: "FPGA"
- board text removed: "FX2MEM"
- board text removed: "G"
- board text removed: "GND"
- board text removed: "Glasgow revC3"
- board text removed: "IO PULL-UP/DOWN"
- board text removed: "LEVEL SHIFTERS"
- board text removed: "LVDS"
- board text removed: "NULL"
- board text removed: "PU/PD A"
- board text removed: "PU/PD B"
- board text removed: "Pull-Up/Down Resistors Bank A"
- board text removed: "Pull-Up/Down Resistors Bank B"
- board text removed: "RECOVER"
- board text removed: "RESET"
- board text removed: "S"
- board text removed: "SEQ"
- board text removed: "STATUS LEDS"
- board text removed: "SYNC"
- board text removed: "U1"
- board text removed: "U2"
- board text removed: "U3"
- board text removed: "U4"
- board text removed: "U5"
- board text removed: "USB FIFO"
- board text removed: "USER LEDS"
- board text removed: "V"
- board text removed: "VDAC"
- board text removed: "VIO A"
- board text removed: "VIO B"
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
